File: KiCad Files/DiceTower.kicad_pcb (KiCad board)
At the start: 2 copper layers, 2 parts, among them U1 NHD-0420H1Z

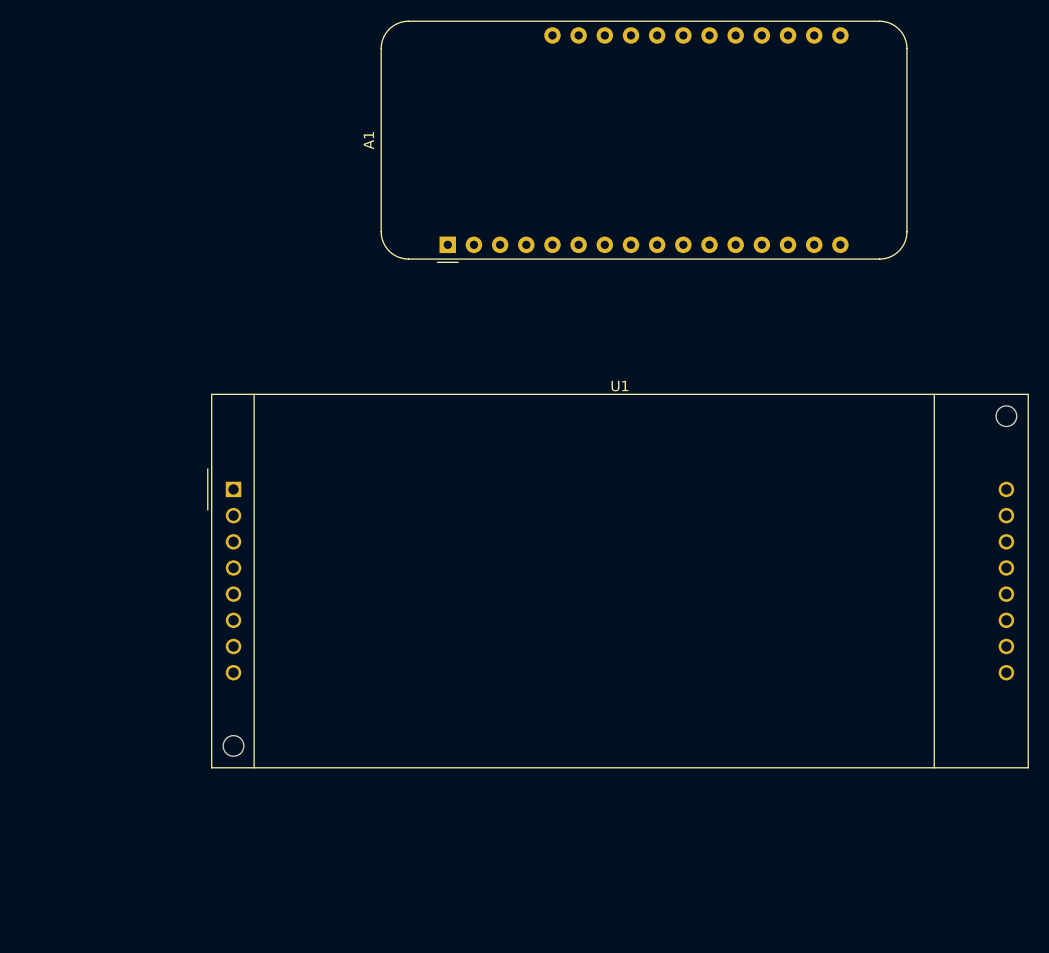
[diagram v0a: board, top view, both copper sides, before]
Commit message: Add PCB
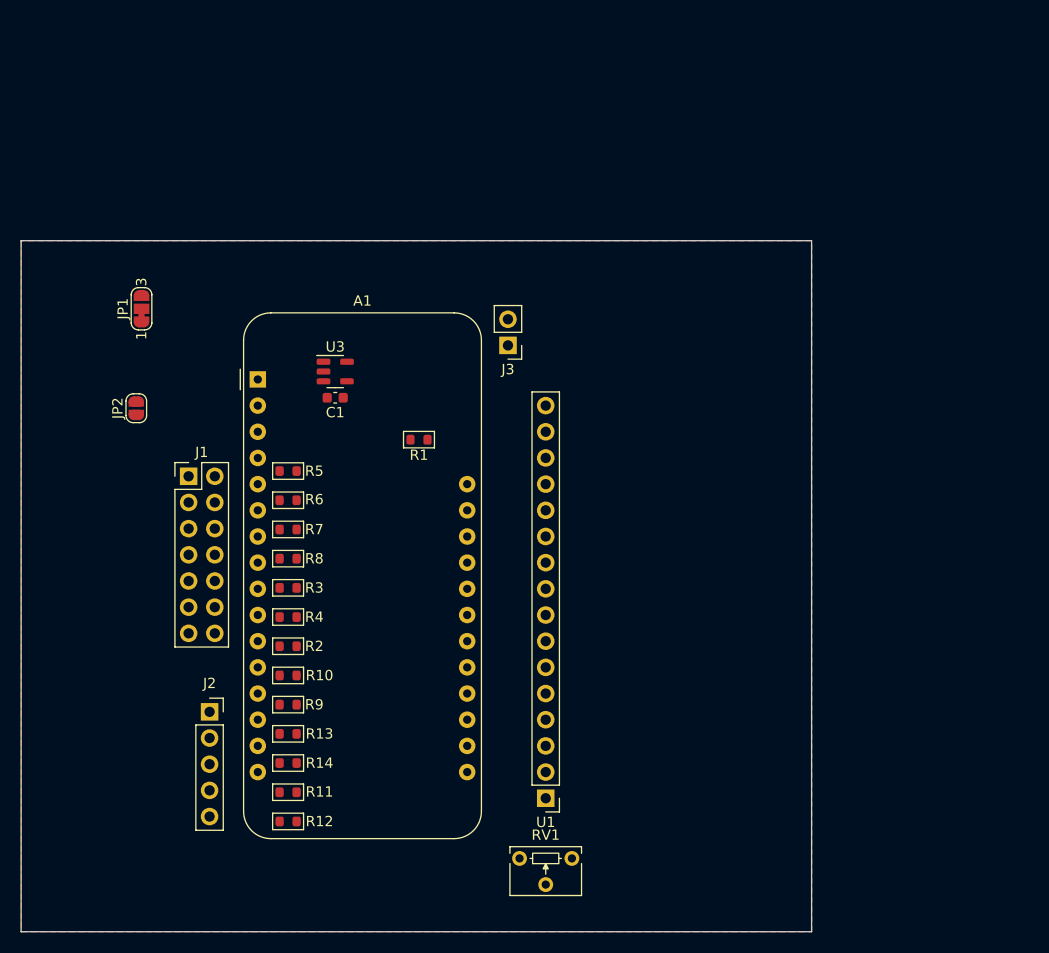
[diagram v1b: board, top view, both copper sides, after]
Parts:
- added C1: 100n, Capacitor_SMD:C_0603_1608Metric, F.Cu at (43.7, 93.5)
- added J1: Conn_02x07_Odd_Even, Connector_PinHeader_2.54mm:PinHeader_2x07_P2.54mm_Vertical, F.Cu at (29.5, 101.1)
- added J2: Conn_01x05_Socket, Connector_PinSocket_2.54mm:PinSocket_1x05_P2.54mm_Vertical, F.Cu at (31.5, 124.0)
- added J3: Conn_01x02_Pin, Connector_PinHeader_2.54mm:PinHeader_1x02_P2.54mm_Vertical, F.Cu at (60.5, 88.4)
- added JP1: Vfeather/Vbatt, Jumper:SolderJumper-3_P1.3mm_Bridged12_RoundedPad1.0x1.5mm_NumberLabels, F.Cu at (24.9, 84.8)
- added JP2: SolderJumper_2_Open, Jumper:SolderJumper-2_P1.3mm_Open_RoundedPad1.0x1.5mm, F.Cu at (24.4, 94.5)
- added R1: 220, PCM_Resistor_SMD_AKL:R_0603_1608Metric, F.Cu at (51.8, 97.5)
- added R10: 10k, PCM_Resistor_SMD_AKL:R_0603_1608Metric, F.Cu at (39.1, 120.4)
- added R11: 10k, PCM_Resistor_SMD_AKL:R_0603_1608Metric, F.Cu at (39.1, 131.8)
- added R12: 18k, PCM_Resistor_SMD_AKL:R_0603_1608Metric, F.Cu at (39.1, 134.6)
- added R13: 10k, PCM_Resistor_SMD_AKL:R_0603_1608Metric, F.Cu at (39.1, 126.1)
- added R14: 18k, PCM_Resistor_SMD_AKL:R_0603_1608Metric, F.Cu at (39.1, 128.9)
- added R2: 10k, PCM_Resistor_SMD_AKL:R_0603_1608Metric, F.Cu at (39.1, 117.6)
- added R3: 10k, PCM_Resistor_SMD_AKL:R_0603_1608Metric, F.Cu at (39.1, 111.9)
- added R4: 10k, PCM_Resistor_SMD_AKL:R_0603_1608Metric, F.Cu at (39.1, 114.8)
- added R5: 10k, PCM_Resistor_SMD_AKL:R_0603_1608Metric, F.Cu at (39.1, 100.6)
- added R6: 10k, PCM_Resistor_SMD_AKL:R_0603_1608Metric, F.Cu at (39.1, 103.4)
- added R7: 10k, PCM_Resistor_SMD_AKL:R_0603_1608Metric, F.Cu at (39.1, 106.3)
- added R8: 10k, PCM_Resistor_SMD_AKL:R_0603_1608Metric, F.Cu at (39.1, 109.1)
- added R9: 18k, PCM_Resistor_SMD_AKL:R_0603_1608Metric, F.Cu at (39.1, 123.3)
- added RV1: R_Potentiometer_Trim, PCM_Potentiometer_THT_AKL:Potentiometer_Bourns_3266W_Vertical, F.Cu at (66.7, 138.2)
- added U3: TPS73131DBV, Package_TO_SOT_SMD:SOT-23-5, F.Cu at (43.7, 90.9)
- U1: footprint Display:NHD-0420H1Z -> Connector_PinHeader_2.54mm:PinHeader_1x16_P2.54mm_Vertical
- moved U1 42.6 mm to (64.1, 132.3), turned to 180 degrees
- moved A1 22.6 mm to (36.2, 91.7), turned to 0 degrees
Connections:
- A1 pad 10: unconnected-(A1-IO4/A5-Pad10) -> /SW2
- A1 pad 11: Net-(A1-SCK/IO5) -> unconnected-(A1-SCK/IO5-Pad11)
- A1 pad 12: Net-(A1-MOSI/IO18) -> /SW0
- A1 pad 13: Net-(A1-MISO/IO19) -> /S2
- A1 pad 14: unconnected-(A1-RX/IO16-Pad14) -> /S1
- A1 pad 15: unconnected-(A1-TX/IO17-Pad15) -> Net-(A1-TX/IO17)
- A1 pad 17: unconnected-(A1-SDA/IO23-Pad17) -> Net-(A1-SDA/IO23)
- A1 pad 18: /DB2 -> Net-(A1-SCL/IO22)
- A1 pad 19: /DB3 -> /DB5
- A1 pad 2: unconnected-(A1-3V3-Pad2) -> +3.3V
- A1 pad 21: /DB5 -> unconnected-(A1-A8/IO15-Pad21)
- A1 pad 24: /DB1 -> unconnected-(A1-A11/IO12-Pad24)
- A1 pad 25: /DB0 -> unconnected-(A1-A12/IO13-Pad25)
- A1 pad 26: +5V -> unconnected-(A1-USB-Pad26)
- A1 pad 27: unconnected-(A1-EN-Pad27) -> Net-(A1-EN)
- A1 pad 28: unconnected-(A1-VBAT-Pad28) -> Net-(A1-VBAT)
- A1 pad 5: unconnected-(A1-DAC2/A0-Pad5) -> /SW3
- A1 pad 6: unconnected-(A1-DAC1/A1-Pad6) -> /SW4
- A1 pad 7: unconnected-(A1-I34/A2-Pad7) -> /SW5
- A1 pad 8: unconnected-(A1-I39/A3-Pad8) -> /SW6
- A1 pad 9: unconnected-(A1-IO36/A4-Pad9) -> /SW1
- U1 pad 10: /DB3 -> unconnected-(U1-DB3-Pad10)
- U1 pad 15: +5V -> +3.3V
- U1 pad 2: +5V -> Net-(JP1-C)
- U1 pad 3: +5V -> Net-(U1-VO)
- U1 pad 4: Net-(A1-SCK/IO5) -> Net-(A1-TX/IO17)
- U1 pad 5: Net-(A1-MOSI/IO18) -> Net-(A1-SDA/IO23)
- U1 pad 6: Net-(A1-MISO/IO19) -> Net-(A1-SCL/IO22)
- U1 pad 7: /DB0 -> unconnected-(U1-DB0-Pad7)
- U1 pad 8: /DB1 -> unconnected-(U1-DB1-Pad8)
- U1 pad 9: /DB2 -> unconnected-(U1-DB2-Pad9)
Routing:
- added copper zone on F.Cu, net GND
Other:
- board outline added: 76.7 x 67.1 mm
